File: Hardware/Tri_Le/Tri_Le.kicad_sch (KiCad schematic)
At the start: 14 parts, among them J1 8P8C_LED_Shielded, SW1 SW_Push, U1 OKI, U2 Teensy4.1_DEV-16771

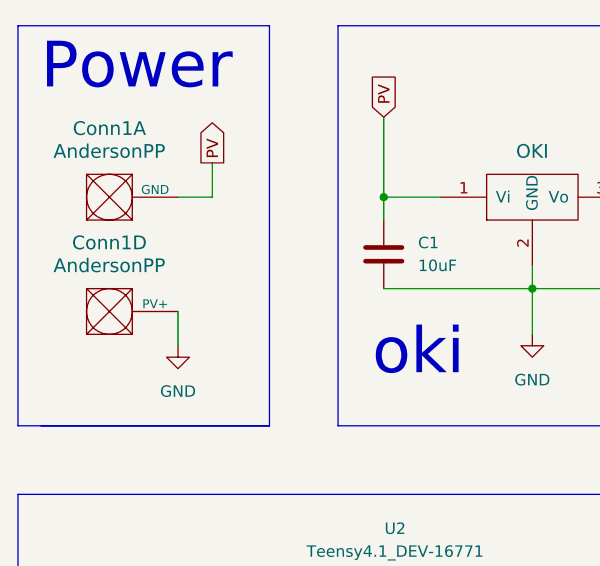
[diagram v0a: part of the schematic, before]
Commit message: Layout Training Finished
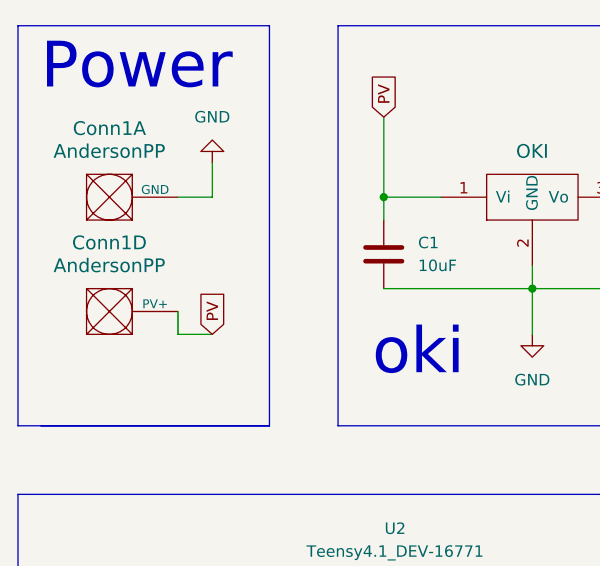
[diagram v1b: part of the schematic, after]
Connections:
- net GND: now also Conn1.1 (GND); no longer Conn1.4 (PV+)
- net PV: now also Conn1.4 (PV+); no longer Conn1.1 (GND)
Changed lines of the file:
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@@
-    (stroke (width 0) (type default))
-  )
-  (wire (pts (xy 36.83 48.26) (xy 36.83 52.07))
     (stroke (width 0) (type default))
   )
@@
     (stroke (width 0) (type default))
   )
+  (wire (pts (xy 40.64 50.8) (xy 36.83 50.8))
+    (stroke (width 0) (type default))
+  )
   (polyline (pts (xy 91.44 68.58) (xy 130.81 68.58))
     (stroke (width 0) (type default))
@@
   )
   (wire (pts (xy 109.22 118.11) (xy 109.22 123.19))
+    (stroke (width 0) (type default))
+  )
+  (wire (pts (xy 36.83 50.8) (xy 36.83 48.26))
     (stroke (width 0) (type default))
   )
@@
     )
   )
-  (global_label "PV" (shape output) (at 40.64 31.75 90) (fields_autoplaced)
-    (effects (font (size 1.27 1.27)) (justify left))
-    (property "Intersheetrefs" "${INTERSHEET_REFS}" (at 40.64 26.4062 90)
-      (effects (font (size 1.27 1.27)) (justify left) hide)
-    )
-  )
   (global_label "PV" (shape input) (at 59.69 26.67 90) (fields_autoplaced)
     (effects (font (size 1.27 1.27)) (justify left))
@@
     (effects (font (size 1.27 1.27)) (justify left))
     (property "Intersheetrefs" "${INTERSHEET_REFS}" (at 147.32 74.6662 90)
+      (effects (font (size 1.27 1.27)) (justify left) hide)
+    )
+  )
+  (global_label "PV" (shape input) (at 40.64 50.8 90) (fields_autoplaced)
+    (effects (font (size 1.27 1.27)) (justify left))
+    (property "Intersheetrefs" "${INTERSHEET_REFS}" (at 40.64 45.4562 90)
       (effects (font (size 1.27 1.27)) (justify left) hide)
     )
@@
     )
   )
-  (symbol (lib_id "power:GND") (at 36.83 52.07 0) (unit 1)
-    (in_bom yes) (on_board yes) (dnp no) (fields_autoplaced)
-    (property "Reference" "#PWR01" (at 36.83 58.42 0)
-      (effects (font (size 1.27 1.27)) hide)
-    )
-    (property "Value" "GND" (at 36.83 57.15 0)
-      (effects (font (size 1.27 1.27)))
-    )
-    (property "Footprint" "" (at 36.83 52.07 0)
-      (effects (font (size 1.27 1.27)) hide)
-    )
-    (property "Datasheet" "" (at 36.83 52.07 0)
-      (effects (font (size 1.27 1.27)) hide)
-    )
-    (pin "1")
-    (instances
-      (project "Tri_Le"
-        (path "/5ff2dd35-a02d-43f5-a1e6-f0bee5eb4477"
-          (reference "#PWR01") (unit 1)
-        )
-      )
-    )
-  )
   (symbol (lib_id "power:+3V3") (at 86.36 78.74 0) (unit 1)
     (in_bom yes) (on_board yes) (dnp no) (fields_autoplaced)
@@
         )
       )
+    )
+  )
+  (symbol (lib_id "power:GND") (at 40.64 31.75 180) (unit 1)
+    (in_bom yes) (on_board yes) (dnp no) (fields_autoplaced)
+    (property "Reference" "#PWR01" (at 40.64 25.4 0)
+      (effects (font (size 1.27 1.27)) hide)
+    )
+    (property "Value" "GND" (at 40.64 26.67 0)
+      (effects (font (size 1.27 1.27)))
+    )
+    (property "Footprint" "" (at 40.64 31.75 0)
+      (effects (font (size 1.27 1.27)) hide)
+    )
+    (property "Datasheet" "" (at 40.64 31.75 0)
+      (effects (font (size 1.27 1.27)) hide)
+    )
+    (pin "1")
+    (instances
+      (project "Tri_Le"
+        (path "/5ff2dd35-a02d-43f5-a1e6-f0bee5eb4477"
+          (reference "#PWR01") (unit 1)
+        )
+      )
